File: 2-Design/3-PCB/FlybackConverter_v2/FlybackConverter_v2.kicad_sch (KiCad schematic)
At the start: 55 parts, among them U1 TL431DBV, U2 LM7812_TO220

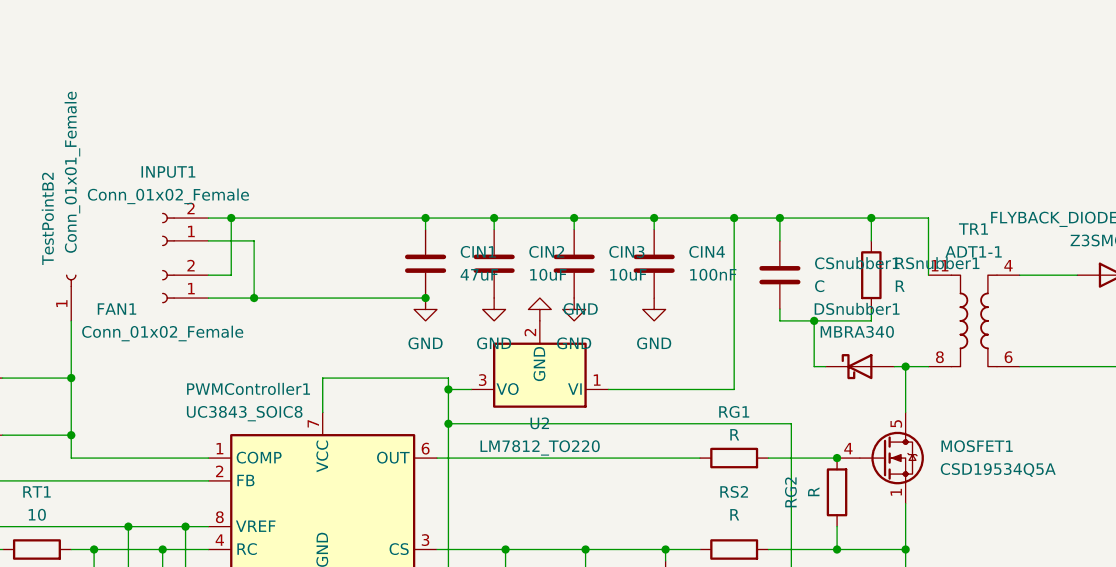
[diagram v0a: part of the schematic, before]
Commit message: I guess, only last edits left for PCB design.
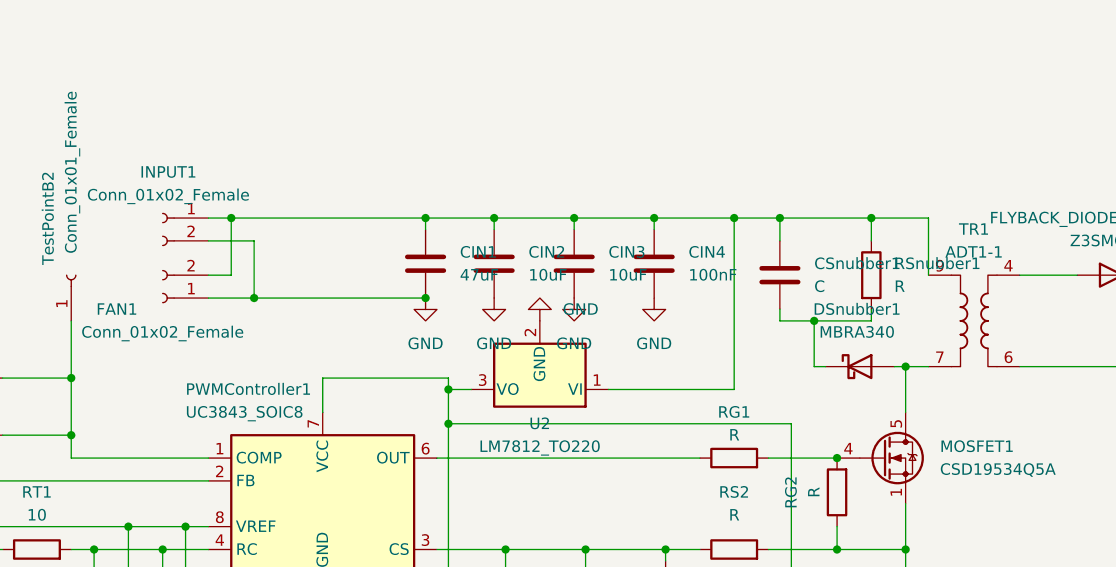
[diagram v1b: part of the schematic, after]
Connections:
- net GND: now also INPUT1.2 (Pin_2); no longer INPUT1.1 (Pin_1)
- net at CIN1.1, CIN2.1, CIN3.1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: now also INPUT1.1 (Pin_1), TR1.9; no longer INPUT1.2 (Pin_2), TR1.11
- net at DSnubber1.2 (A), MOSFET1.5 (D): now also TR1.7; no longer TR1.8
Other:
- moved on the sheet: INPUT1
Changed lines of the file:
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@@
     (pin "5")
   )
-  (symbol (lib_id "Connector:Conn_01x02_Female") (at 97.79 40.64 180) (unit 1)
+  (symbol (lib_id "Connector:Conn_01x02_Female") (at 97.79 38.1 0) (mirror y) (unit 1)
     (in_bom yes) (on_board yes) (fields_autoplaced)
     (property "Reference" "INPUT1" (id 0) (at 98.425 33.02 0))
     (property "Value" "Conn_01x02_Female" (id 1) (at 98.425 35.56 0))
-    (property "Footprint" "kutup:sevgi_konnektosu" (id 2) (at 97.79 40.64 0)
-      (effects (font (size 1.27 1.27)) hide)
-    )
-    (property "Datasheet" "~" (id 3) (at 97.79 40.64 0)
+    (property "Footprint" "kutup:sevgi_konnektosu" (id 2) (at 97.79 38.1 0)
+      (effects (font (size 1.27 1.27)) hide)
+    )
+    (property "Datasheet" "~" (id 3) (at 97.79 38.1 0)
       (effects (font (size 1.27 1.27)) hide)
     )
@@
       (effects (font (size 1.27 1.27)) hide)
     )
-    (pin "11")
+    (pin "9")
     (pin "4")
     (pin "6")
-    (pin "8")
+    (pin "7")
   )
   (symbol (lib_id "Device:R") (at 207.01 69.85 0) (unit 1)
